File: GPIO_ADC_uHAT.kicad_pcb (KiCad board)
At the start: 2 copper layers, 65 x 30.5 mm, 17 parts, among them J1 rpi_uhat_sym, J2 Conn_01x10, J3 Conn_01x10, J4 Conn_01x08, J5 Conn_01x02, U1 MCP23017_SO, U3 CAT24C128, U4 MCP3208

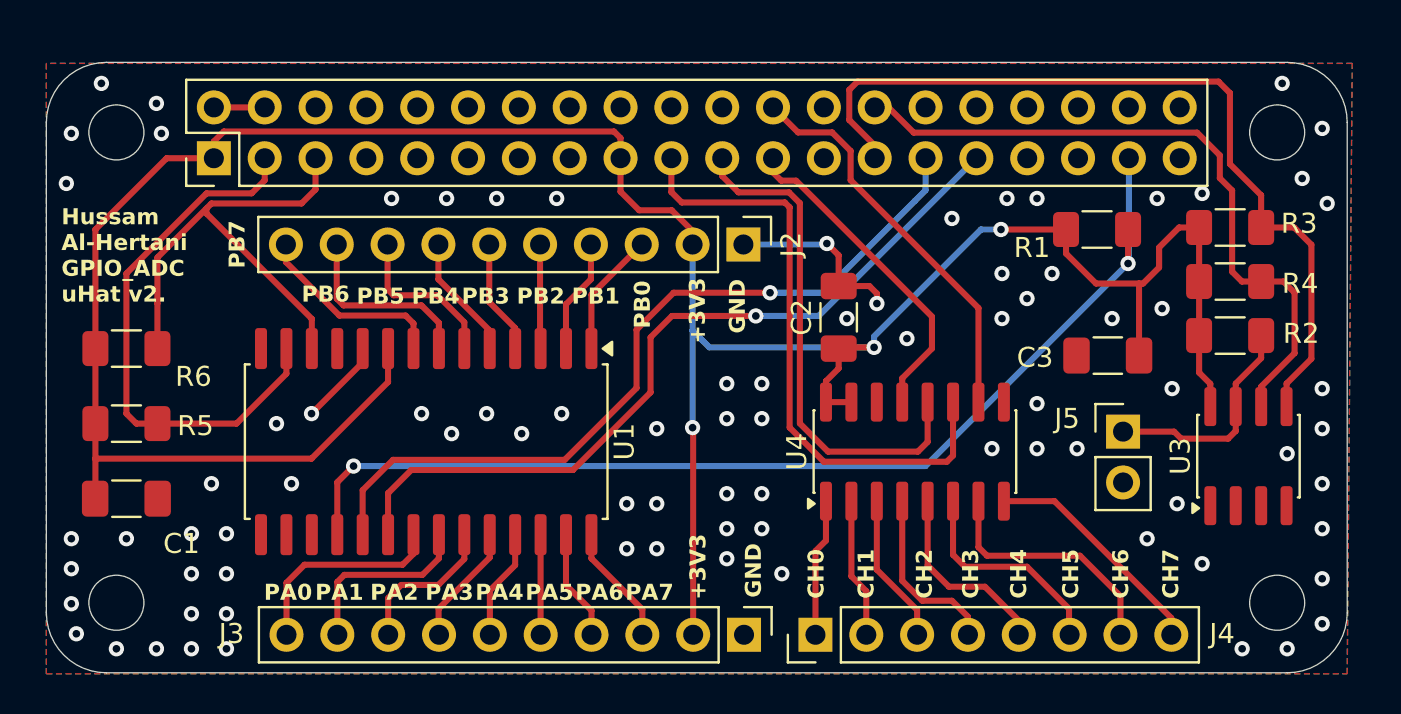
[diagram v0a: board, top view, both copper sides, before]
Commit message: made some modifications and added test code
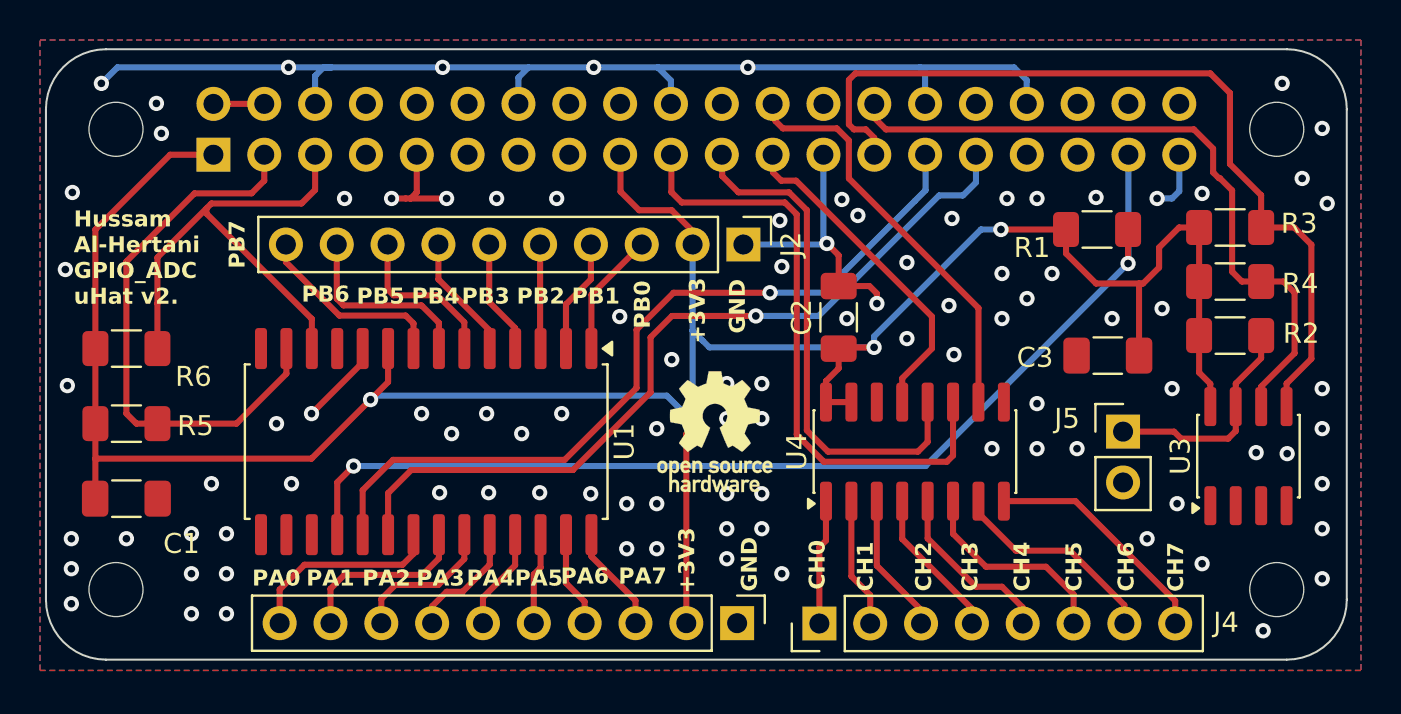
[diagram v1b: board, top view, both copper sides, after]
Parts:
- added REF**: OSHW-Logo_5.7x6mm_SilkScreen, Symbol:OSHW-Logo_5.7x6mm_SilkScreen, F.Cu at (150.4, 77.4)
- J1: footprint myparts:rpi_uhat_fpt -> myparts:rpi_uhat_fpt_v2
- moved J1 40.0 mm to (116.9, 97.4)
- moved J3 0.67 mm to (151.5, 87.0)
- moved J4 0.60 mm to (155.6, 87.0)
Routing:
- net GND: track 13.4 -> 83.3 mm, vias 84 -> 98
- net +3V3: track 138.4 -> 132.2 mm, vias 3 -> 4
- net /CH6: track 12.3 -> 10.7 mm
- net /CH3: track 8.91 -> 7.55 mm
- net /GPA3: track 6.07 -> 7.13 mm
- net INTA: track 40.0 -> 40.9 mm
- net ID_SDA: track 42.2 -> 43.0 mm
- net /CH4: track 9.62 -> 8.84 mm
- net /GPA6: track 5.53 -> 4.81 mm
- net /GPA7: track 6.05 -> 5.33 mm
- net CE0: track 20.0 -> 20.6 mm
- net /CH0: track 6.89 -> 6.25 mm
- net /CH5: track 10.9 -> 10.4 mm
- net ID_SCL: track 34.2 -> 34.8 mm
- net SDA: track 27.4 -> 28.0 mm
